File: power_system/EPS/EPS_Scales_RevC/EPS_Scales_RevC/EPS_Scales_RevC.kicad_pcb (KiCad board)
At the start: 4 copper layers, 95.2 x 66 mm, 252 parts, among them J1 Input Power, J10 DF11-16DP-2DSA, J11 DN-T1-GE3_VIS, J12 DF11-16DP-2DSA, J15 DN-T1-GE3_VIS, J16 Conn_01x04, J18 Conn_01x04, J2 Conn_01x01_Socket, J3 Conn_01x01_Socket, J4 Conn_01x01_Socket, J5 Conn_01x01_Socket, J6 DF11-16DP-2DSA, J7 DN-T1-GE3_VIS, J8 Conn_01x04, U1 LTC4365, U10 LTC4365, U11 LT8638S, U12 INA230, U13 TLV1704, U14 TLV1704, U2 LT8638SEVPBF, U3 INA230, U4 TLV1704, U5 LTC4365, U6 LT8638S, U7 LTC6902, U8 INA230, U9 LTC4300A-1

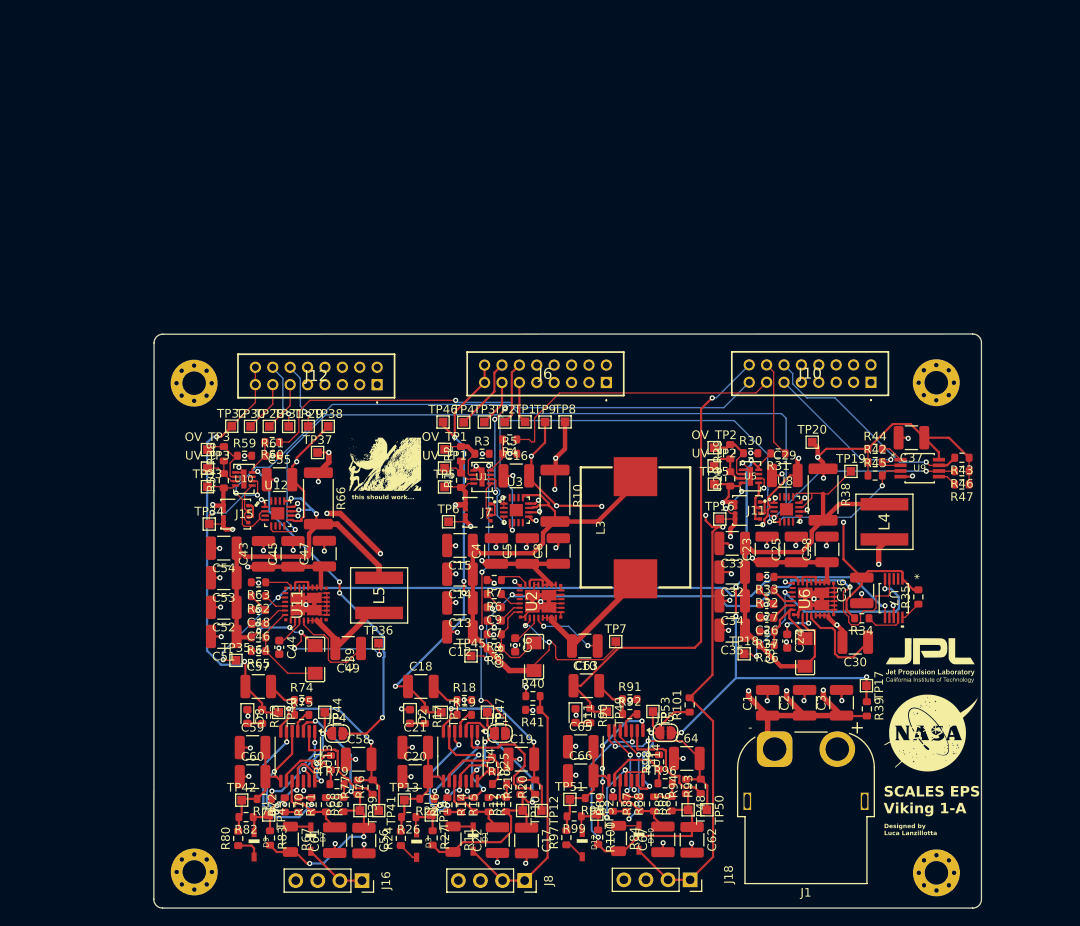
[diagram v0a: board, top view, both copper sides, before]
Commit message: Revert "Luca branch v2"
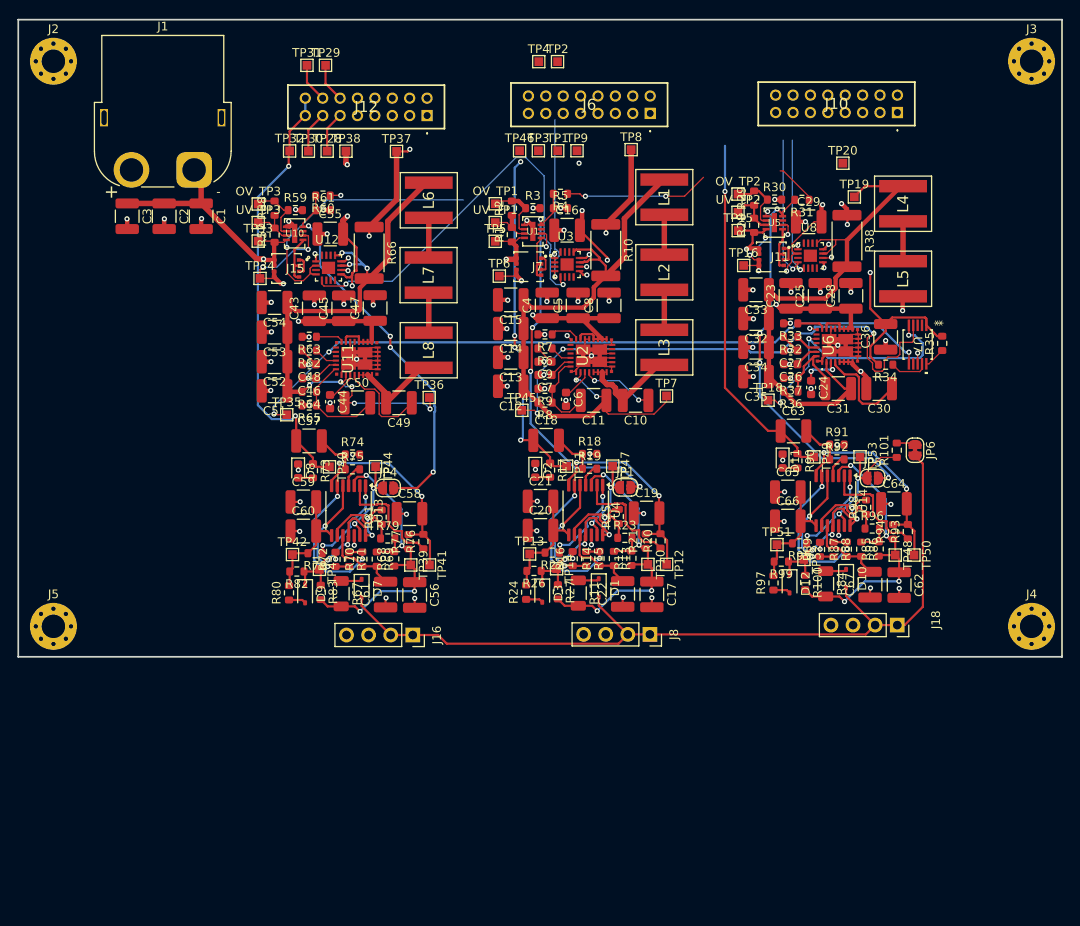
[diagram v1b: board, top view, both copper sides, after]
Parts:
- removed C37: 10n, Capacitor_SMD:C_1210_3225Metric
- removed C38, C39: 22p, easyeda2kicad:C1206
- removed G*** (x3): LOGO, LOGO
- removed R39: 100k, Resistor_SMD:R_0603_1608Metric
- removed R40: 150k, Resistor_SMD:R_0603_1608Metric
- removed R41: 50k, Resistor_SMD:R_0603_1608Metric
- removed R42, R43, R44, R45, R46, R47: 10k, Resistor_SMD:R_0603_1608Metric
- removed TP17: TestPoint, TestPoint:TestPoint_Pad_1.0x1.0mm
- removed U9: LTC4300A-1, RevC Footprints:LTC4300A-1
- added C11: 22p, Capacitor_SMD:C_1210_3225Metric, F.Cu at (152.1, 64.8)
- added C50: 22p, Capacitor_SMD:C_1210_3225Metric, F.Cu at (125.0, 65.0)
- added JP6: SolderJumper_2_Open, Jumper:SolderJumper-2_P1.3mm_Open_RoundedPad1.0x1.5mm, F.Cu at (189.1, 70.5)
- added L1: 3.3u, RevC Footprints:XEL6030102MEC, F.Cu at (160.3, 41.4)
- added L2: 3.3u, RevC Footprints:XEL6030102MEC, F.Cu at (160.3, 50.0)
- added L6: 1u, RevC Footprints:XEL6030102MEC, F.Cu at (133.2, 41.8)
- added L7: 1u, RevC Footprints:XEL6030102MEC, F.Cu at (133.2, 50.4)
- added L8: 1u, RevC Footprints:XEL6030102MEC, F.Cu at (133.2, 59.0)
- C31: footprint easyeda2kicad:C1206 -> Capacitor_SMD:C_1210_3225Metric
- D1, D10, D12, D3, D7, D9: footprint RevC Footprints:SODFL2512X100N -> Diode_SMD:D_SOD-323
- L3: value 10u -> 3.3u; footprint easyeda2kicad:IND-SMD_L13.8-W12.6_MHCC12050 -> RevC Footprints:XEL6030102MEC
- L4: value 2.2u -> 1u; footprint RevC Footprints:XEL6030 -> RevC Footprints:XEL6030102MEC
- L5: value 3.3u -> 1u; footprint RevC Footprints:XEL6030 -> RevC Footprints:XEL6030102MEC
- R31: value 100k -> 1k
- R65, R9: value 3.0k -> 3k
- moved C3 99.4 mm to (98.5, 43.6), turned to -90 degrees
- moved J1 94.3 mm to (106.2, 38.3), turned to 0 degrees
- moved C2 92.5 mm to (102.8, 43.6), turned to -90 degrees
- moved C1 85.9 mm to (107.0, 43.6), turned to -90 degrees
- moved L5 70.4 mm to (187.7, 50.8)
- moved TP4 42.4 mm to (145.8, 25.8)
- moved TP2 41.9 mm to (148.0, 25.8)
- moved TP31 41.6 mm to (119.2, 26.2)
- moved TP29 41.6 mm to (121.3, 26.2)
- moved J2 40.4 mm to (90.0, 25.8)
- moved J3 38.5 mm to (202.5, 25.8)
- moved D12 38.3 mm to (174.7, 85.9)
- moved D10 38.2 mm to (181.2, 85.3)
- moved C62 37.7 mm to (187.3, 86.0)
- moved R96 37.7 mm to (184.2, 79.5)
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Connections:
- D1 pad 2: +5V_WD_J -> +5V_Perif
- D10 pad 2: +3.3V_OBC -> +5V_Perif
- J18 pad 1: +3.3V_OBC -> +5V_Perif
- J18 pad 2: +3.3V_OBC -> +5V_Perif
- J8 pad 1: +5V_WD_J -> +5V_Perif
- J8 pad 2: +5V_WD_J -> +5V_Perif
- L3 pad 2: Net-(U2-BIAS) -> Net-(L2-Pad1)
- L4 pad 1: Net-(U6-SW) -> Net-(L4-Pad1)
- L5 pad 1: Net-(U11-SW) -> Net-(U6-SW)
- L5 pad 2: Net-(U11-BIAS) -> Net-(L4-Pad1)
- R101 pad 2: +3.3V_OBC -> +5V_Perif
- U12 pad 2: SDA -> OBC SDA
- U12 pad 4: SDA -> OBC SDA
- U12 pad 5: SCL -> OBC SCL
- U3 pad 4: SDA -> OBC SDA
- U3 pad 5: SCL -> OBC SCL
- U8 pad 4: SDA -> OBC SDA
- U8 pad 5: SCL -> OBC SCL
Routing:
- net +3.3V_OBC: track 238.2 -> 97.2 mm
- net SDA: track 126.5 -> 0.00 mm, vias 6 -> 0
- net SCL: track 113.6 -> 0.00 mm, vias 4 -> 0
- net ~{OBC_Toggle_Perif}: track 59.0 -> 1.24 mm
- net OBC SDA: track 19.3 -> 67.7 mm, vias 1 -> 3
- net +5V_Perif: track 84.2 -> 130.6 mm, vias 5 -> 3
- net +20V_Jetson: track 56.0 -> 15.4 mm, vias 4 -> 2
- net OBC SCL: track 25.5 -> 63.8 mm, vias 1 -> 3
- net +V_Batt: track 143.8 -> 108.1 mm, vias 6 -> 3
- net +5V_WD_J: track 30.0 -> 0.00 mm
- net ~{OBC_Toggle_Jetson}: track 33.3 -> 16.6 mm, vias 0 -> 2
- net WDT_WDI_OBC: track 56.6 -> 41.7 mm
- net WDT_WDI_Jetson: track 51.3 -> 39.7 mm
- net ~{WD_TOGGLE_OBC}: track 57.7 -> 46.2 mm, vias 5 -> 4
- net GND: track 167.3 -> 157.7 mm, vias 93 -> 90
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- removed copper zone on In2.Cu, net +V_Batt
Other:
- board size 95.2 x 66 mm -> 120 x 73.2 mm
- board text removed: "Designed by Luca Lanzillotta"
- board text removed: "SCALES EPS Viking 1-A"
- board text removed: "this should work..."

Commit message: Update EPS_Scales_RevC.kicad_pcb
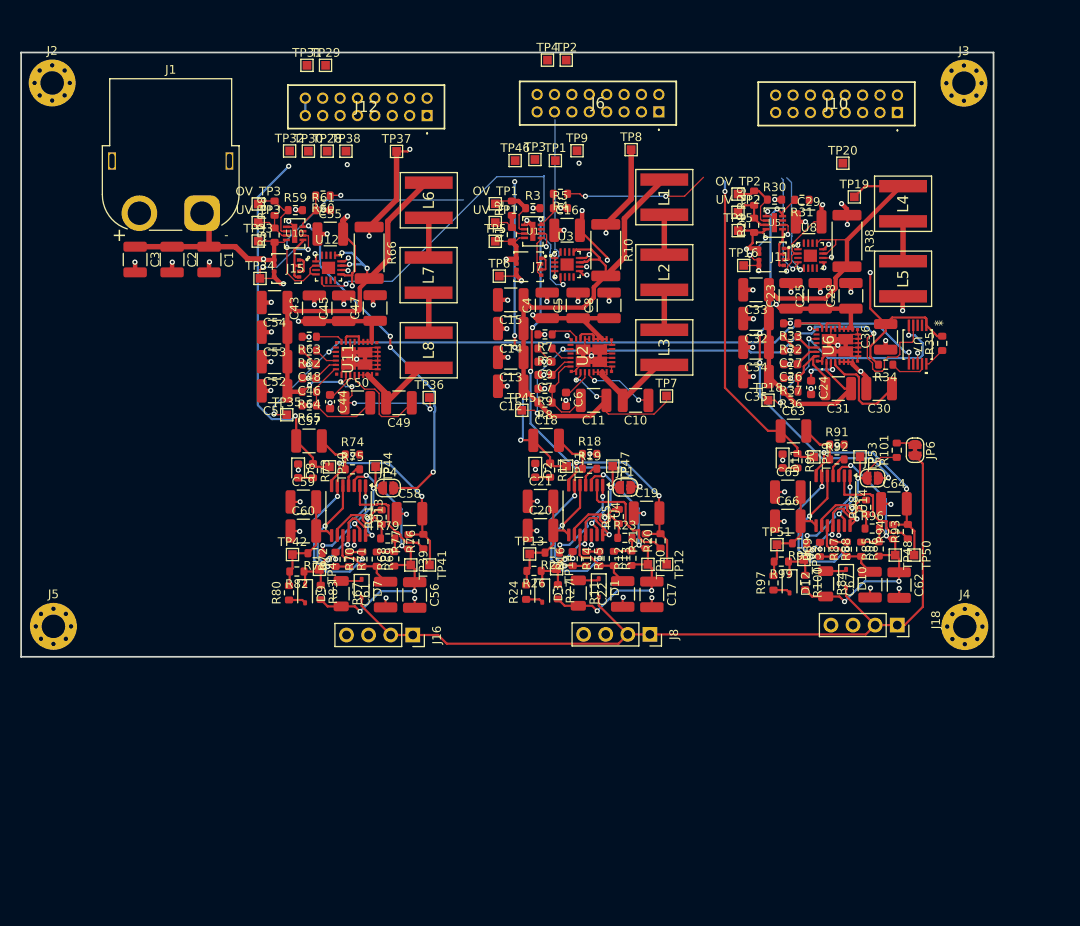
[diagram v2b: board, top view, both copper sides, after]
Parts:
- moved J3 8.17 mm to (194.7, 28.3)
- moved J4 7.68 mm to (194.8, 90.8)
- moved J1 5.06 mm to (107.1, 43.2)
- moved C1 5.06 mm to (107.9, 48.6)
- moved C2 5.06 mm to (103.7, 48.6)
- moved C3 5.06 mm to (99.4, 48.6)
- moved J2 2.50 mm to (89.9, 28.3)
- moved TP46 1.24 mm to (143.1, 37.2)
- moved TP1 1.16 mm to (147.8, 37.2)
- moved TP3 1.08 mm to (145.4, 37.1)
- moved TP2 1.02 mm to (149.0, 25.6)
- moved TP4 1.02 mm to (146.8, 25.6)
- moved J6 1.02 mm to (159.7, 31.6)
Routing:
- net +5V_Perif: track 130.6 -> 118.7 mm
- net WDT_WDI_Perif: track 50.9 -> 44.5 mm
- net +V_Batt: track 108.1 -> 101.9 mm
- net OBC SCL: track 63.8 -> 58.1 mm
- net Net-(J12-Pad13): track 4.78 -> 0.00 mm
- net Net-(J12-Pad11): track 4.71 -> 0.00 mm
- net ~{OBC_Toggle_OBC}: track 4.92 -> 0.37 mm
- net Net-(J12-Pad14): track 4.52 -> 0.00 mm
- net Net-(J12-Pad12): track 4.47 -> 0.00 mm
- net OBC SDA: track 67.7 -> 63.4 mm
- net WDT_WDI_OBC: track 41.7 -> 37.8 mm
- net WDT_WDI_Jetson: track 39.7 -> 37.1 mm
- net +3.3V_OBC: track 97.2 -> 95.1 mm
- net GND: track 157.7 -> 158.4 mm
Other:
- board size 120 x 73.2 mm -> 111.8 x 69.5 mm
